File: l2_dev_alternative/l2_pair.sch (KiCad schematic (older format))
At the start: 14 parts, among them U1102 NC7WZ17, U201 NC7WZ17, U203 NCP1529, U204 INA219

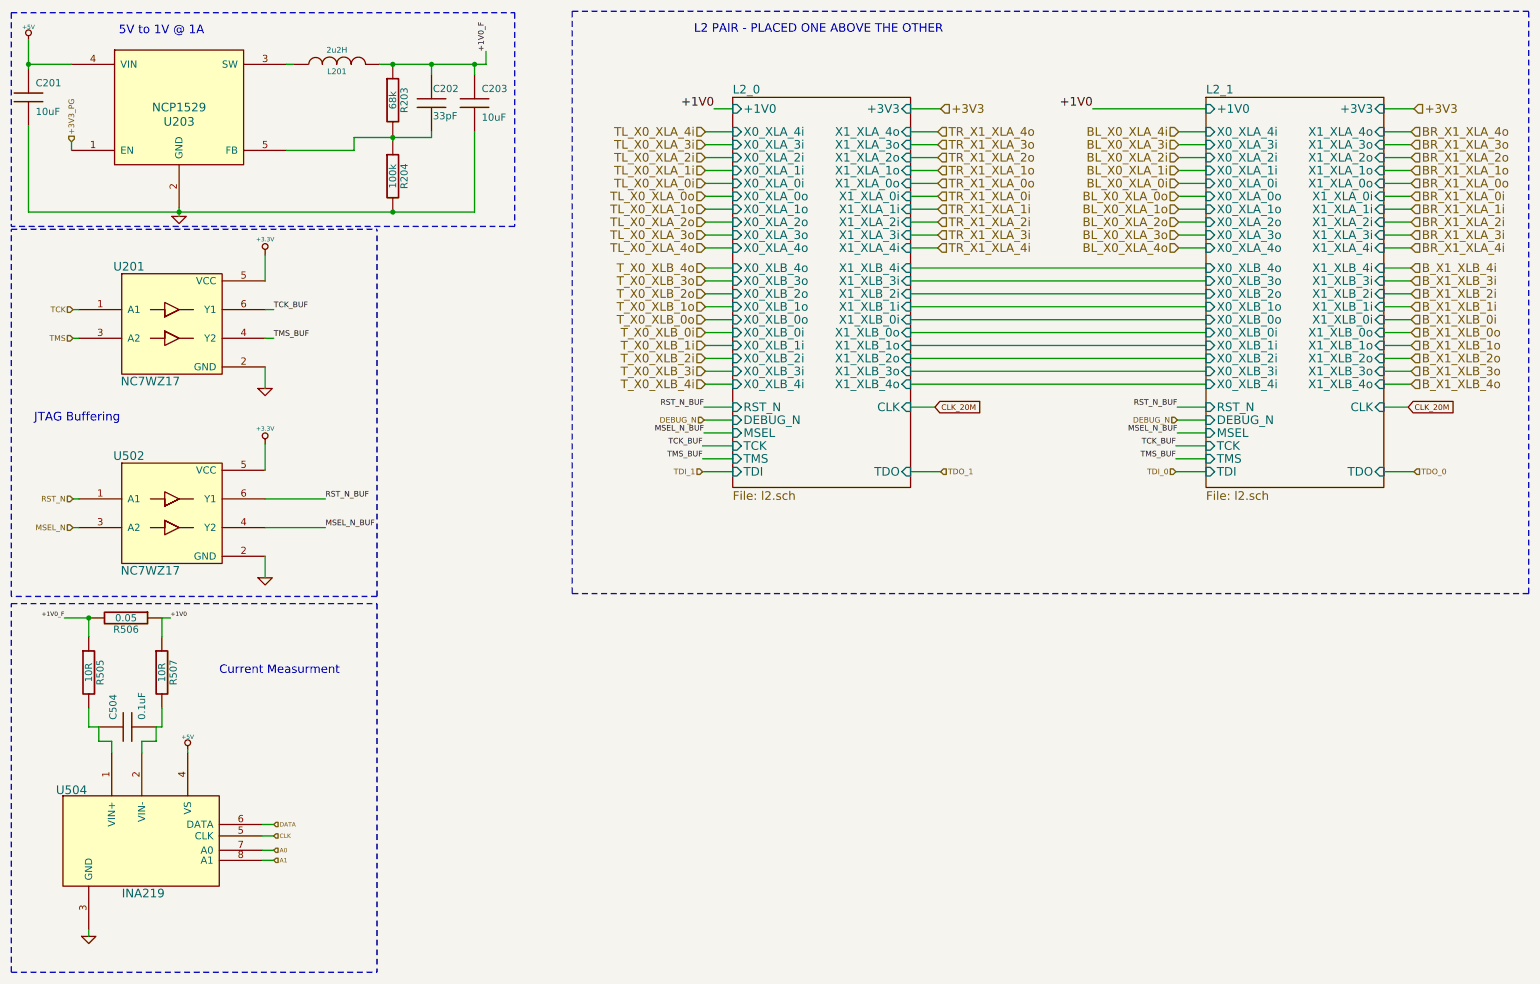
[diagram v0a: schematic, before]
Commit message: Most of the components now in. About to try finalise the size!
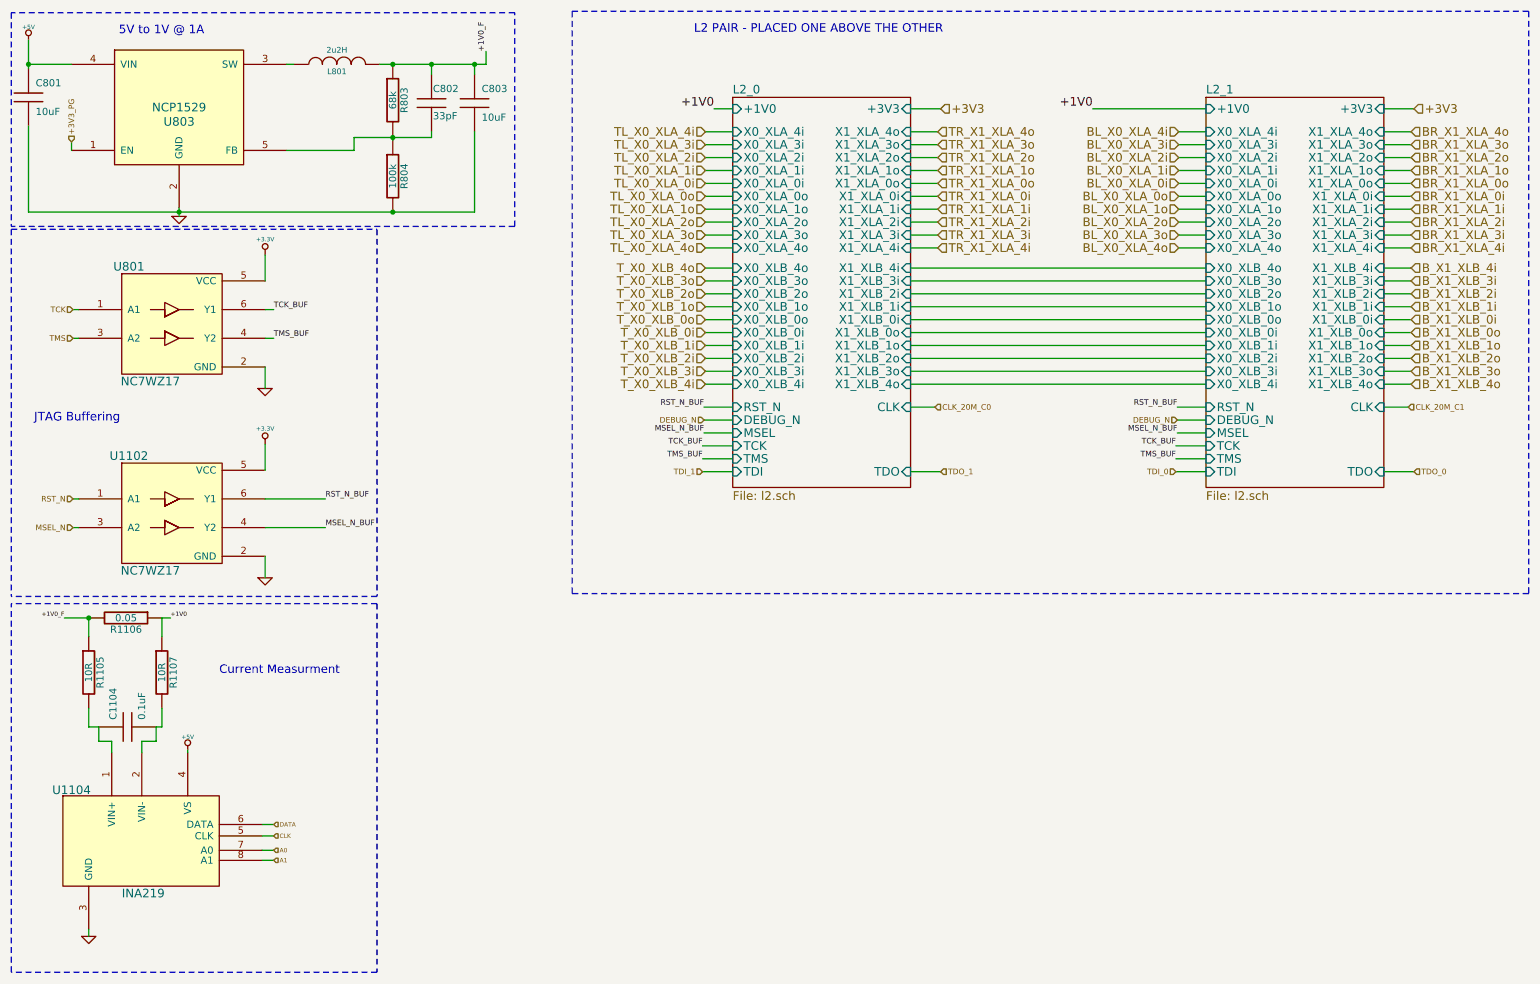
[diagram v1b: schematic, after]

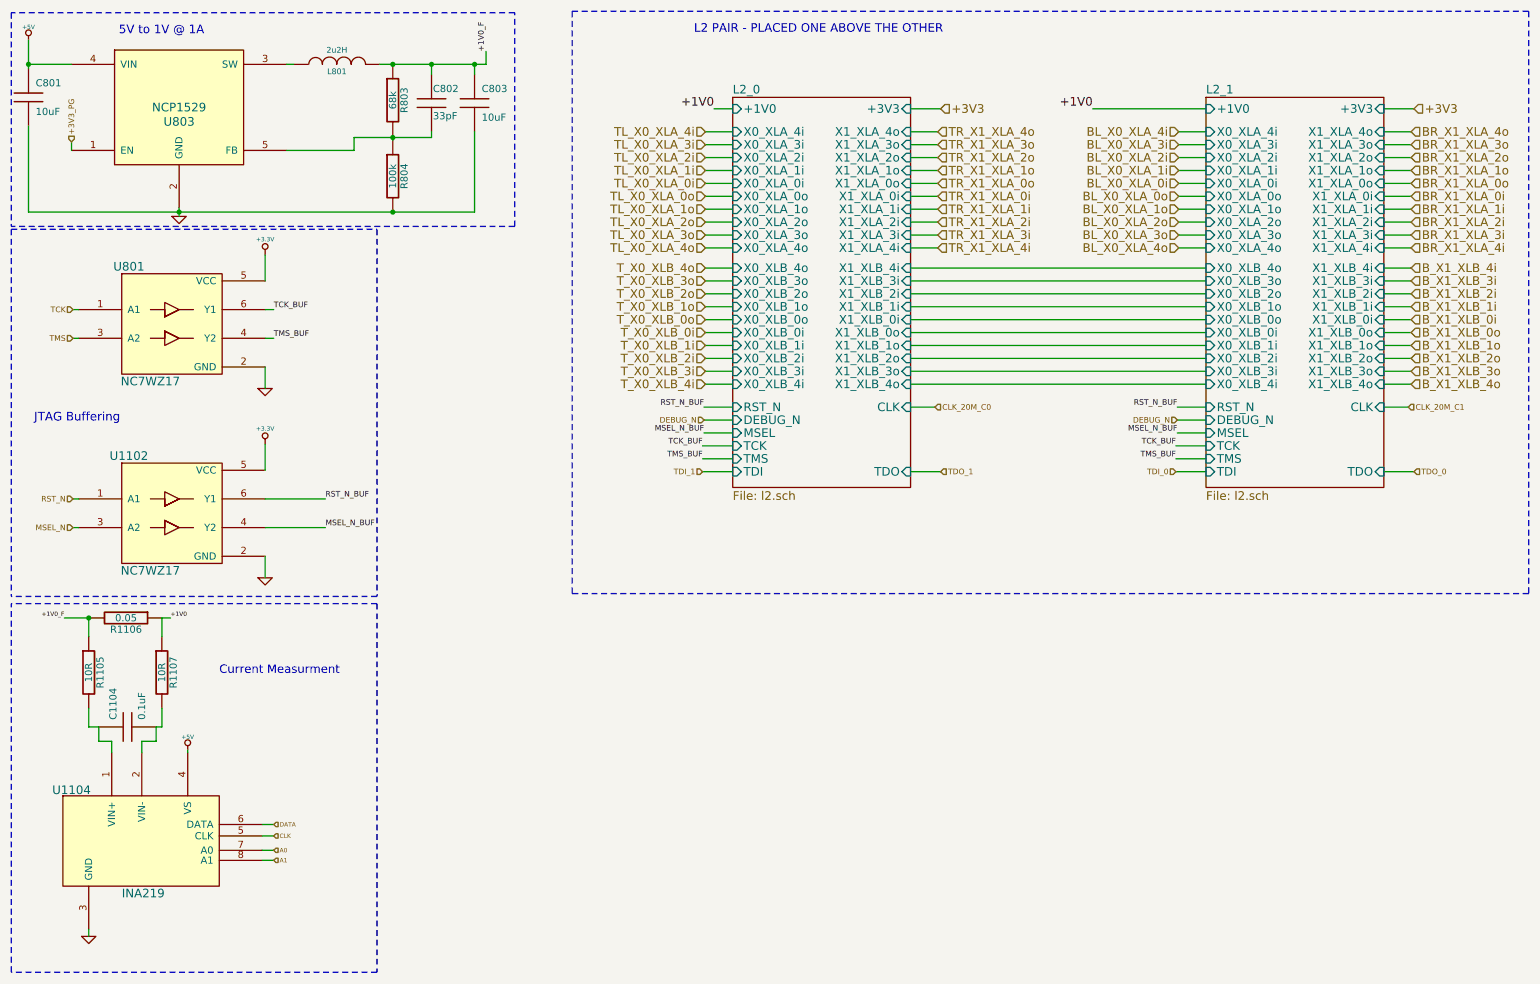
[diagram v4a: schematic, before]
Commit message: need to check if L1 X-linkks need buffering
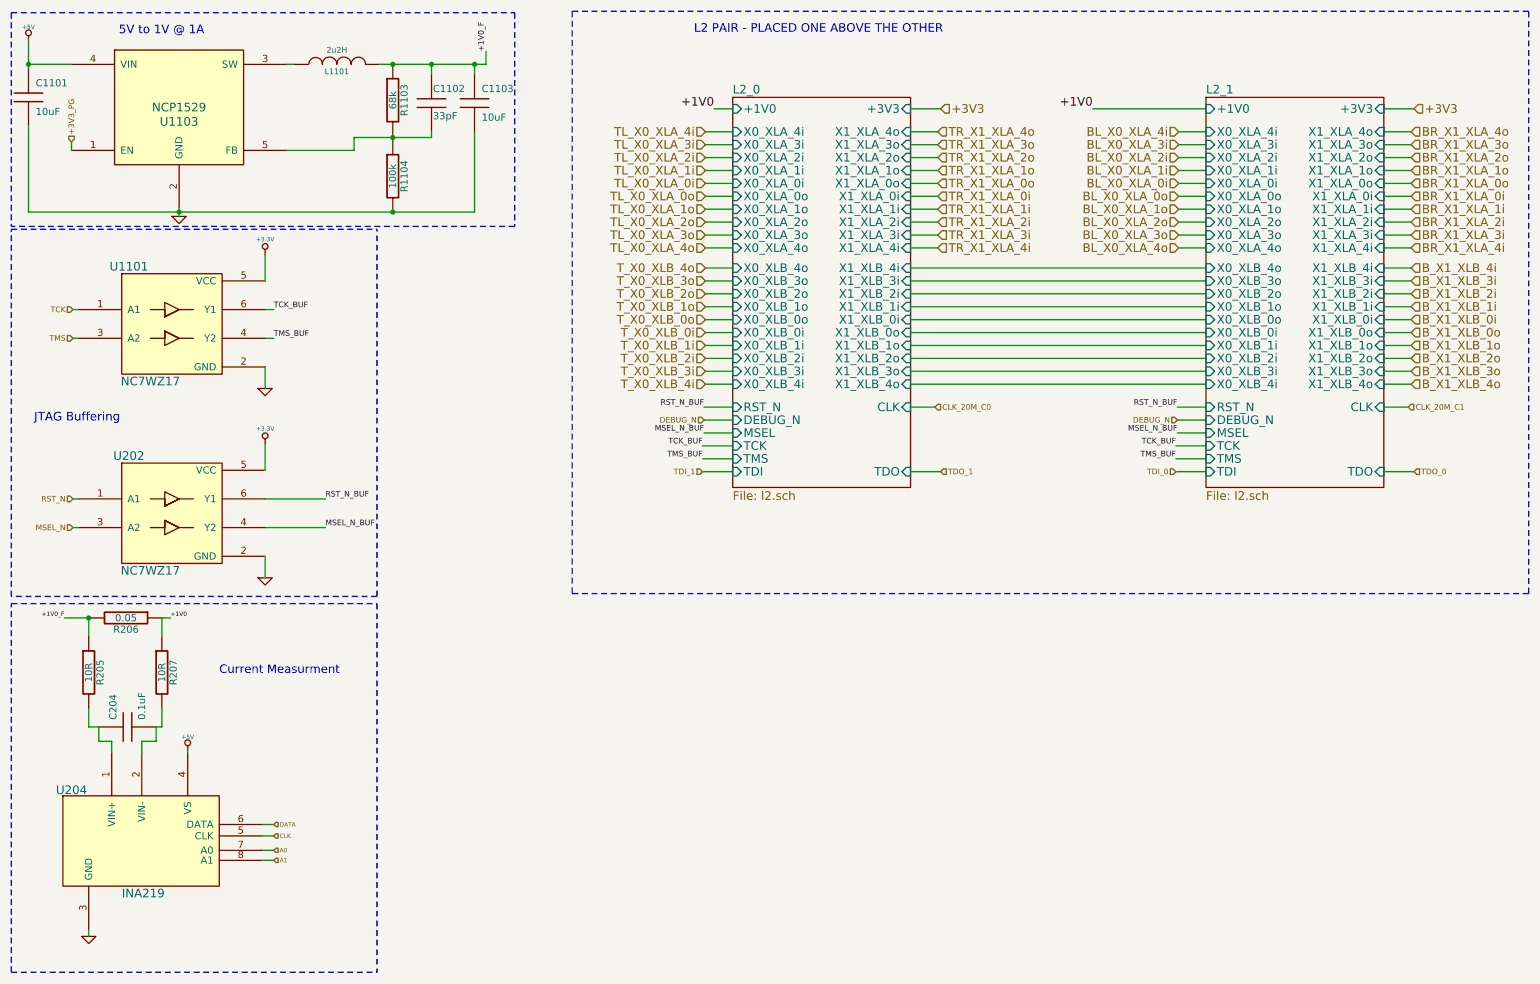
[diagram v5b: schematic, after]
